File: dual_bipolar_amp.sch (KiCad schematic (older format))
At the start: 9 parts, among them U4 OPA2156xD

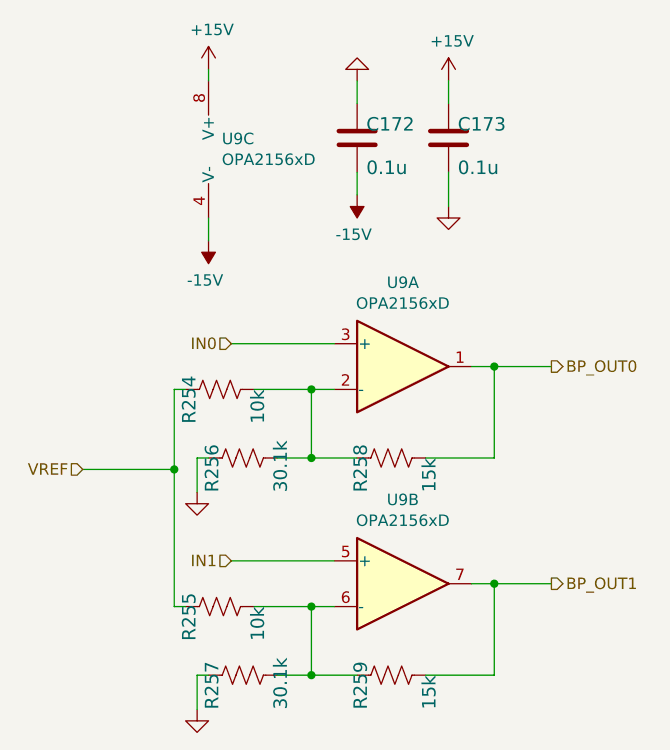
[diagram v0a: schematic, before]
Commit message: before importing autoroute
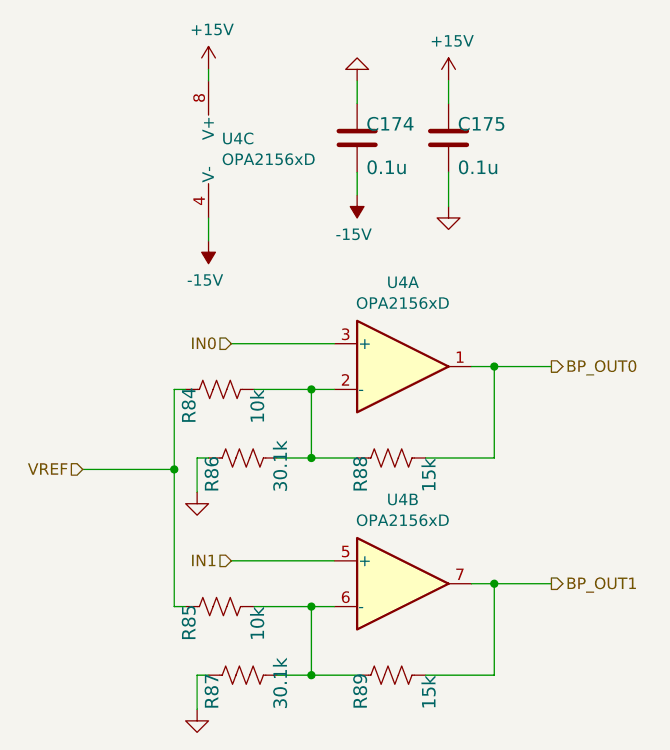
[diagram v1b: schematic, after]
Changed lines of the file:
@@
 $Descr A4 11693 8268
 encoding utf-8
-Sheet 26 26
+Sheet 23 26
 Title ""
 Date ""
@@
 AR Path="/6095BD4C/60EB6FD5/60F31C8B" Ref="U2"  Part="1"
 AR Path="/61B02572/60EB6FD5/60F31C8B" Ref="U9"  Part="1"
-F 0 "U9" H 5600 3617 50  0000 C CNN
+F 0 "U4" H 5600 3617 50  0000 C CNN
 F 1 "OPA2156xD" H 5600 3526 50  0000 C CNN
 F 2 "Package_SO:SOIC-8_3.9x4.9mm_P1.27mm" H 5700 3250 50  0001 C CNN
@@
 AR Path="/6095BD4C/60EB6FD5/60F31C94" Ref="R3"  Part="1"
 AR Path="/61B02572/60EB6FD5/60F31C94" Ref="R254"  Part="1"
-F 0 "R254" H 4650 3450 59  0000 L BNN
+F 0 "R84" H 4650 3450 59  0000 L BNN
 F 1 "10k" H 4650 3150 59  0000 L BNN
 F 2 "Resistor_SMD:R_0603_1608Metric" H 4800 3350 50  0001 C CNN
@@
 AR Path="/6095BD4C/60EB6FD5/60F31C9B" Ref="U2"  Part="3"
 AR Path="/61B02572/60EB6FD5/60F31C9B" Ref="U9"  Part="3"
-F 0 "U9" H 4808 2346 50  0000 L CNN
+F 0 "U4" H 4808 2346 50  0000 L CNN
 F 1 "OPA2156xD" H 4808 2255 50  0000 L CNN
 F 2 "Package_SO:SOIC-8_3.9x4.9mm_P1.27mm" H 4850 2300 50  0001 C CNN
@@
 AR Path="/6095BD4C/60EB6FD5/60F31CA4" Ref="R7"  Part="1"
 AR Path="/61B02572/60EB6FD5/60F31CA4" Ref="R256"  Part="1"
-F 0 "R256" H 4750 3750 59  0000 L BNN
+F 0 "R86" H 4750 3750 59  0000 L BNN
 F 1 "30.1k" H 4750 3450 59  0000 L BNN
 F 2 "Resistor_SMD:R_0603_1608Metric" H 4900 3650 50  0001 C CNN
@@
 AR Path="/6095BD4C/60EB6FD5/60F31CB1" Ref="R13"  Part="1"
 AR Path="/61B02572/60EB6FD5/60F31CB1" Ref="R258"  Part="1"
-F 0 "R258" H 5400 3750 59  0000 L BNN
+F 0 "R88" H 5400 3750 59  0000 L BNN
 F 1 "15k" H 5400 3450 59  0000 L BNN
 F 2 "Resistor_SMD:R_0603_1608Metric" H 5550 3650 50  0001 C CNN
@@
 AR Path="/6095BD4C/60EB6FD5/60F31CB8" Ref="U2"  Part="2"
 AR Path="/61B02572/60EB6FD5/60F31CB8" Ref="U9"  Part="2"
-F 0 "U9" H 5600 4567 50  0000 C CNN
+F 0 "U4" H 5600 4567 50  0000 C CNN
 F 1 "OPA2156xD" H 5600 4476 50  0000 C CNN
 F 2 "Package_SO:SOIC-8_3.9x4.9mm_P1.27mm" H 5700 4200 50  0001 C CNN
@@
 AR Path="/6095BD4C/60EB6FD5/60F31CC1" Ref="R4"  Part="1"
 AR Path="/61B02572/60EB6FD5/60F31CC1" Ref="R255"  Part="1"
-F 0 "R255" H 4650 4400 59  0000 L BNN
+F 0 "R85" H 4650 4400 59  0000 L BNN
 F 1 "10k" H 4650 4100 59  0000 L BNN
 F 2 "Resistor_SMD:R_0603_1608Metric" H 4800 4300 50  0001 C CNN
@@
 AR Path="/6095BD4C/60EB6FD5/60F31CCA" Ref="R8"  Part="1"
 AR Path="/61B02572/60EB6FD5/60F31CCA" Ref="R257"  Part="1"
-F 0 "R257" H 4750 4700 59  0000 L BNN
+F 0 "R87" H 4750 4700 59  0000 L BNN
 F 1 "30.1k" H 4750 4400 59  0000 L BNN
 F 2 "Resistor_SMD:R_0603_1608Metric" H 4900 4600 50  0001 C CNN
@@
 AR Path="/6095BD4C/60EB6FD5/60F31CD7" Ref="R14"  Part="1"
 AR Path="/61B02572/60EB6FD5/60F31CD7" Ref="R259"  Part="1"
-F 0 "R259" H 5400 4700 59  0000 L BNN
+F 0 "R89" H 5400 4700 59  0000 L BNN
 F 1 "15k" H 5400 4400 59  0000 L BNN
 F 2 "Resistor_SMD:R_0603_1608Metric" H 5550 4600 50  0001 C CNN
@@
 AR Path="/6095BD4C/60EB6FD5/60F31CED" Ref="C5"  Part="1"
 AR Path="/61B02572/60EB6FD5/60F31CED" Ref="C172"  Part="1"
-F 0 "C172" H 5440 2275 59  0000 L BNN
+F 0 "C174" H 5440 2275 59  0000 L BNN
 F 1 "0.1u" H 5440 2085 59  0000 L BNN
 F 2 "Capacitor_SMD:C_0603_1608Metric" H 5400 2250 50  0001 C CNN
@@
 AR Path="/6095BD4C/60EB6FD5/60F31CF7" Ref="C6"  Part="1"
 AR Path="/61B02572/60EB6FD5/60F31CF7" Ref="C173"  Part="1"
-F 0 "C173" H 5840 2275 59  0000 L BNN
+F 0 "C175" H 5840 2275 59  0000 L BNN
 F 1 "0.1u" H 5840 2085 59  0000 L BNN
 F 2 "Capacitor_SMD:C_0603_1608Metric" H 5800 2250 50  0001 C CNN
